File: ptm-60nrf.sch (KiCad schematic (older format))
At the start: 24 parts, among them J1 USB_C_Receptacle_USB2.0, J2 BAT, J3 Conn_01x04_Male, J4 SWD, Q1 AO3407, U1 TP4054, U2 XC6220B331MR-G, U3 nRF52840_holyiot_18010, U4 SRV05-4

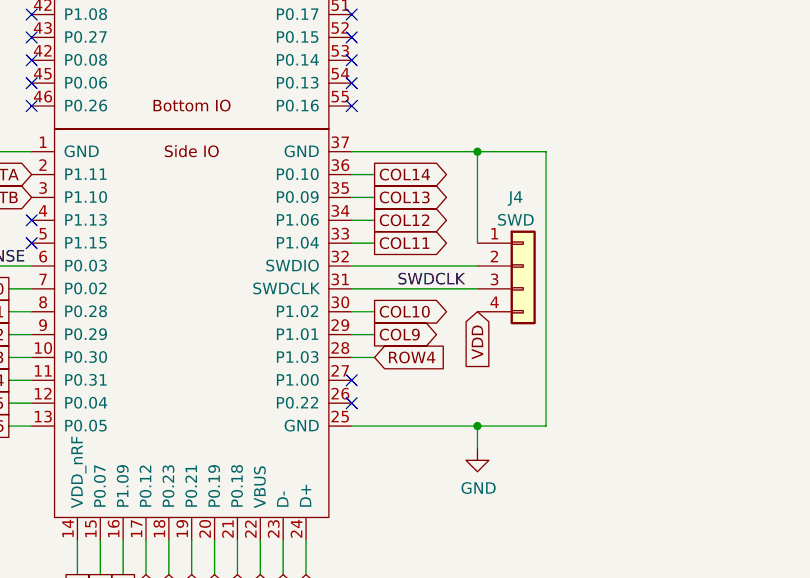
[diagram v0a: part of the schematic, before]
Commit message: updated README
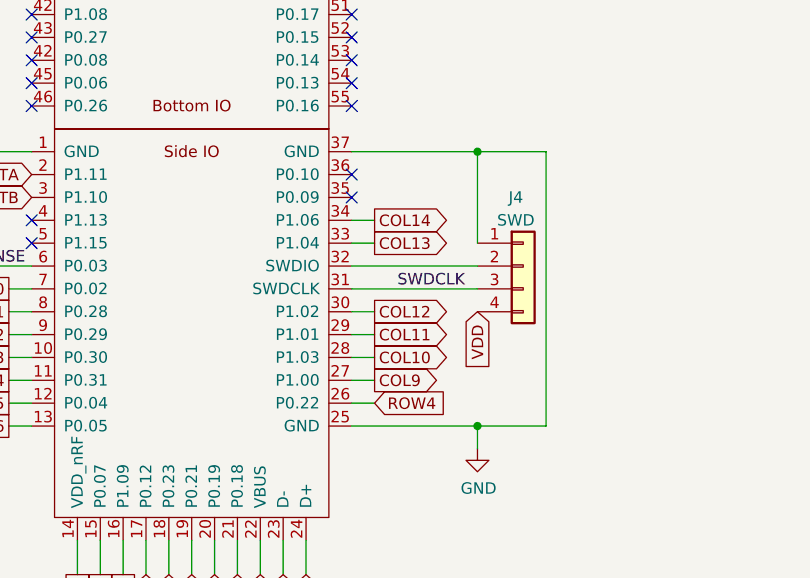
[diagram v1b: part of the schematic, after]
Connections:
- net COL10: now also U3.28 (P1.03); no longer U3.30 (P1.02)
- net COL11: now also U3.29 (P1.01); no longer U3.33 (P1.04)
- net COL12: now also U3.30 (P1.02); no longer U3.34 (P1.06)
- net COL13: now also U3.33 (P1.04); no longer U3.35 (P0.09)
- net COL14: now also U3.34 (P1.06); no longer U3.36 (P0.10)
- net COL9: now also U3.27 (P1.00); no longer U3.29 (P1.01)
- net ROW4: now also U3.26 (P0.22); no longer U3.28 (P1.03)
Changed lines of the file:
@@
 Text GLabel 2800 6650 3    50   Input ~ 0
 ROW3
-Text GLabel 3800 5700 2    50   Input ~ 0
+Text GLabel 3800 5900 2    50   Input ~ 0
 ROW4
-Wire Wire Line
-	3800 4900 3700 4900
-Wire Wire Line
-	3800 5000 3700 5000
 Wire Wire Line
 	3800 5100 3700 5100
@@
 Text GLabel 2700 6650 3    50   Output ~ 0
 COL8
-Wire Wire Line
-	3800 5700 3700 5700
+Text GLabel 3800 5800 2    50   Output ~ 0
+COL9
+Wire Wire Line
+	2200 5400 2300 5400
+Text GLabel 3800 5100 2    50   Output ~ 0
+COL14
+Wire Wire Line
+	2200 5900 2300 5900
+Text GLabel 3800 5200 2    50   Output ~ 0
+COL13
+Wire Wire Line
+	2200 5800 2300 5800
+Text GLabel 3800 5500 2    50   Output ~ 0
+COL12
+Wire Wire Line
+	2200 5700 2300 5700
 Text GLabel 3800 5600 2    50   Output ~ 0
-COL9
-Wire Wire Line
-	2200 5400 2300 5400
-Text GLabel 3800 4900 2    50   Output ~ 0
-COL14
-Wire Wire Line
-	2200 5900 2300 5900
-Text GLabel 3800 5000 2    50   Output ~ 0
-COL13
-Wire Wire Line
-	2200 5800 2300 5800
-Text GLabel 3800 5100 2    50   Output ~ 0
-COL12
-Wire Wire Line
-	2200 5700 2300 5700
-Text GLabel 3800 5200 2    50   Output ~ 0
 COL11
 Wire Wire Line
 	2200 5600 2300 5600
-Text GLabel 3800 5500 2    50   Output ~ 0
+Text GLabel 3800 5700 2    50   Output ~ 0
 COL10
 Wire Wire Line
@@
 NoConn ~ 3700 4500
 NoConn ~ 3700 4600
-NoConn ~ 3700 5800
-NoConn ~ 3700 5900
 NoConn ~ 4500 1900
 NoConn ~ 4300 1900
@@
 Text GLabel 6900 1600 2    50   Input ~ 0
 VB
+Wire Wire Line
+	3800 5700 3700 5700
+Wire Wire Line
+	3800 5800 3700 5800
+Wire Wire Line
+	3800 5900 3700 5900
+NoConn ~ 3700 5000
+NoConn ~ 3700 4900
 $EndSCHEMATC
